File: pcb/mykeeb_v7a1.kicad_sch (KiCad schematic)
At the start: 71 parts, among them SW43 SW_Push, SW44 SW_SPDT, U1 74HC595, U2 xiao-ble

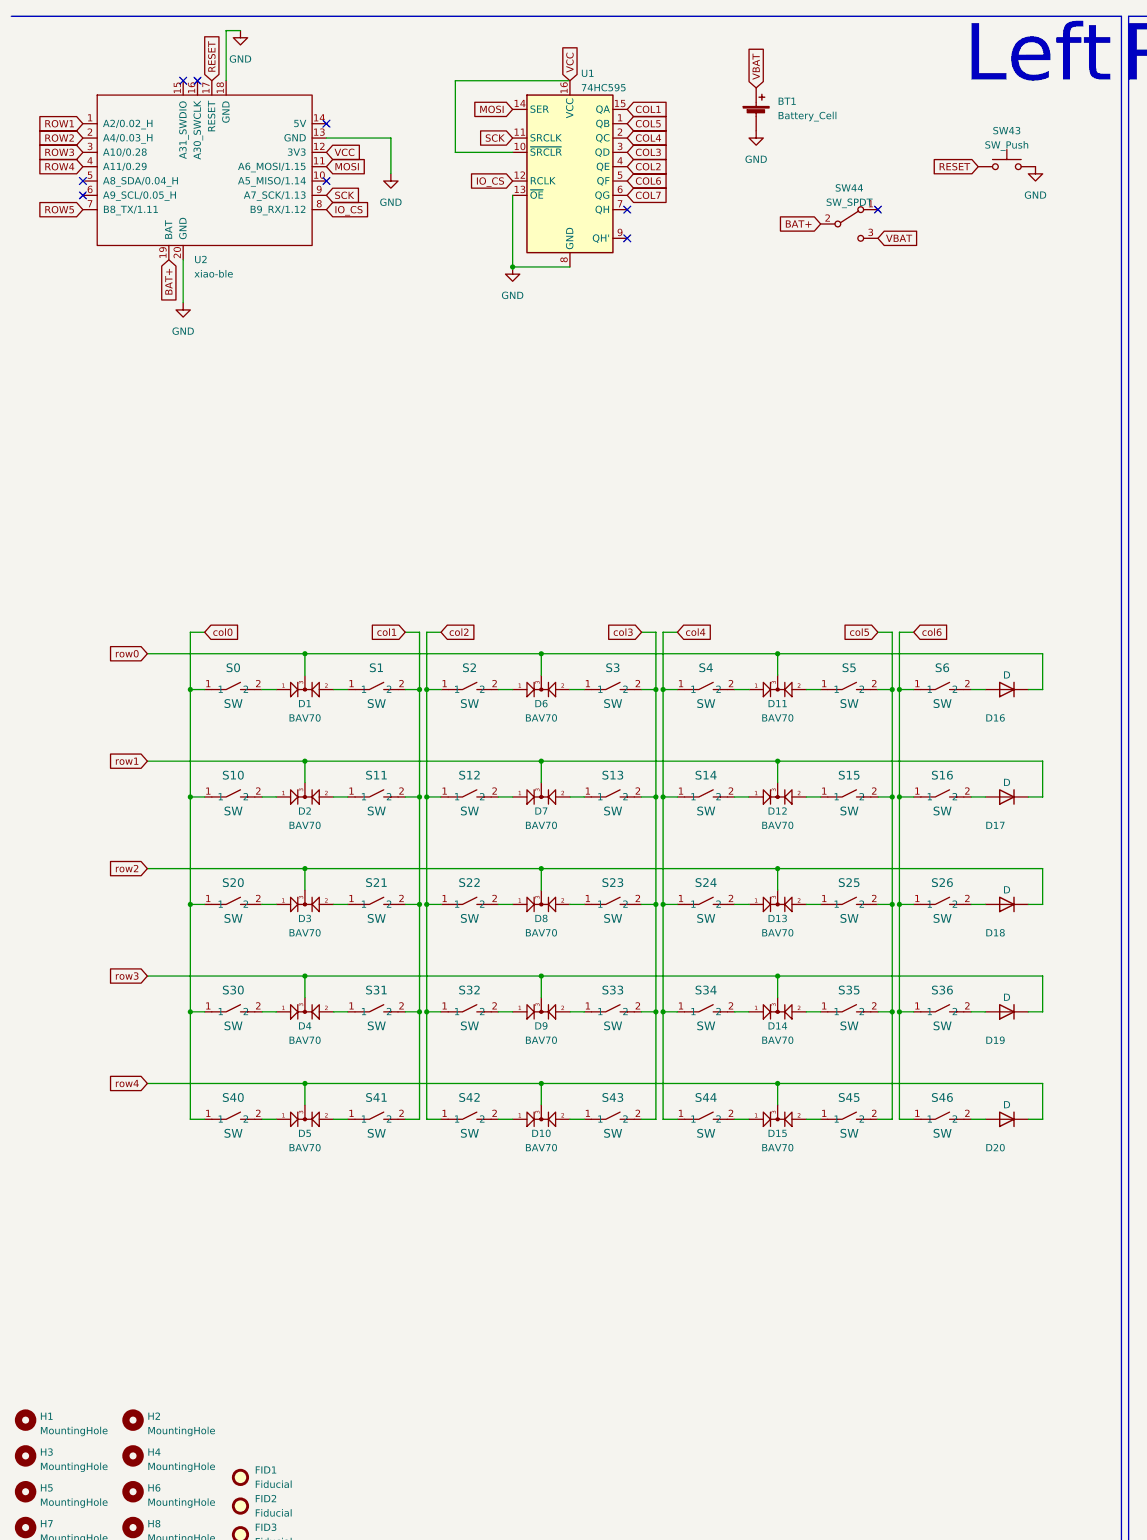
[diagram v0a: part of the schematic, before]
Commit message: wip
Signed-off-by: Maximilian Huber <gh@maxhbr.de>
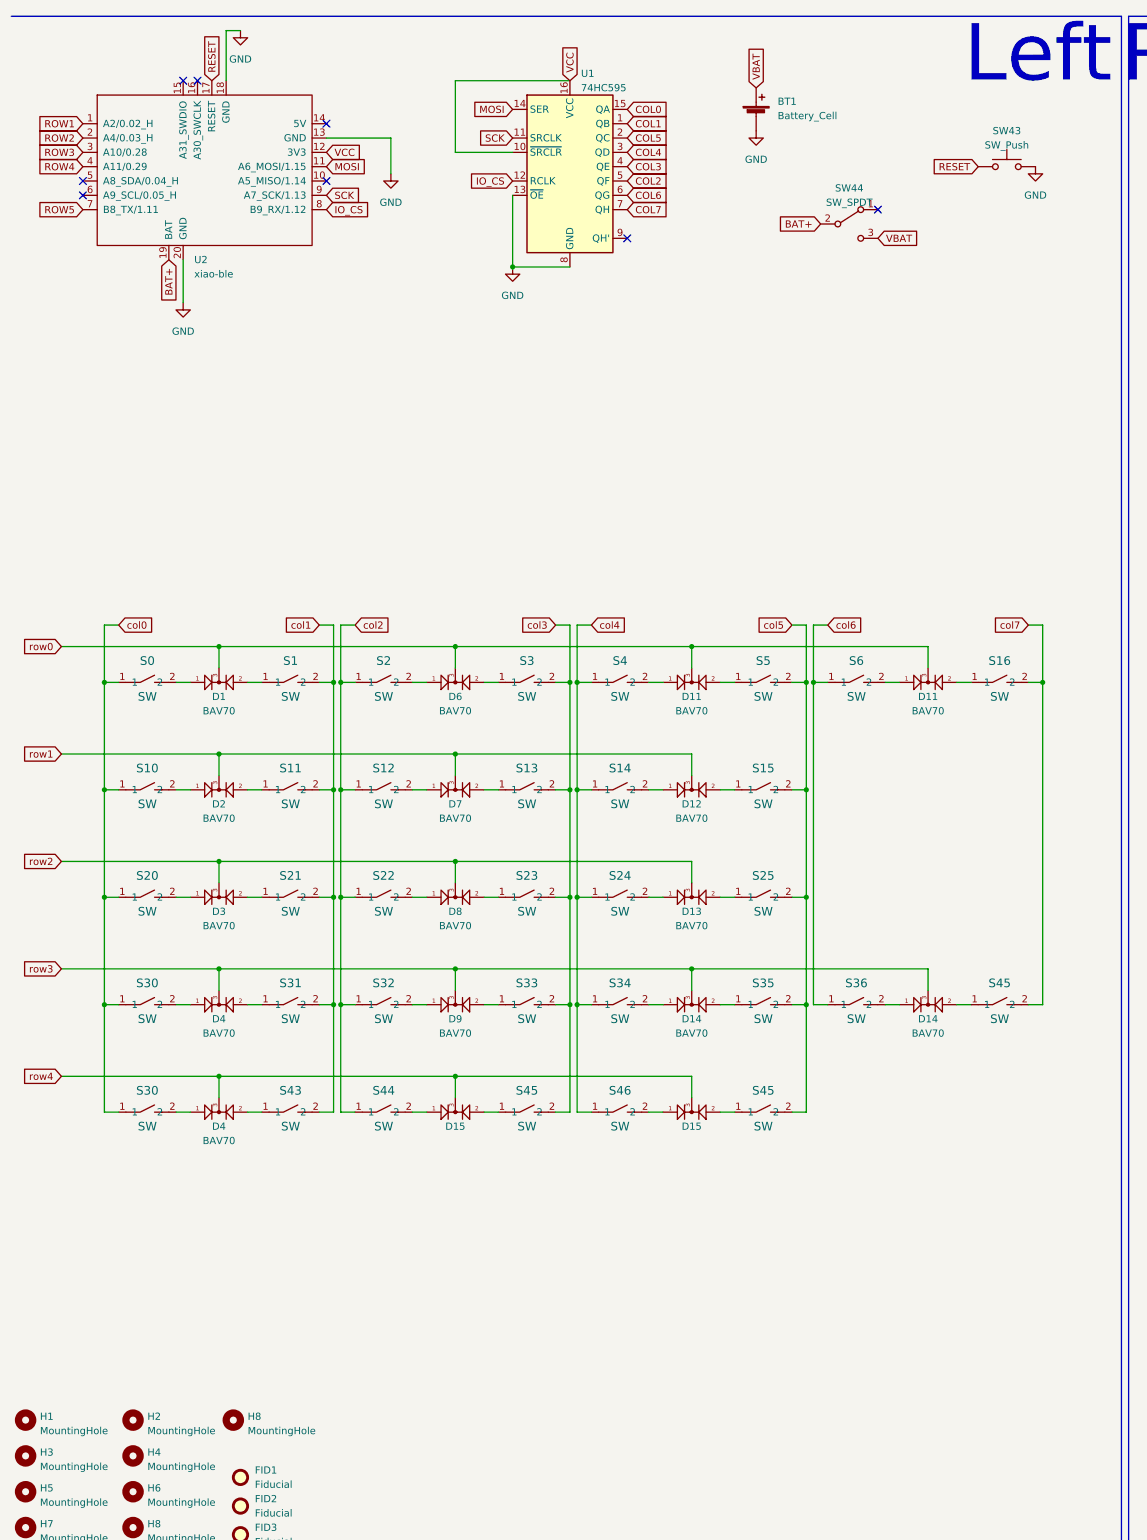
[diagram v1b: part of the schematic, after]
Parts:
- removed D10, D5: BAV70, mykeeb:SOT-23, symbol hillside_basic:BAV70_Small
- removed D16, D17, D18, D19, D20: D, mykeeb:D3_SMD, symbol Device:D
- removed S26, S40, S41, S42: SW, mykeeb:MX_KAILH_SOCKET_1U, symbol YAEMK:MX_1U
- added D11, D14, D15, D4: BAV70, Package_TO_SOT_SMD:SOT-23, symbol hillside_basic:BAV70_Small
- added H8: MountingHole, MountingHole:MountingHole_2.2mm_M2_DIN965, symbol Mechanical:MountingHole
- added S30, S45 (x2): SW, pretty:MX-1U-Hotswap, symbol YAEMK:MX_1U
- D1, D11, D12, D13, D14, D15, D2, D3, D4, D6, D7, D8, D9: footprint mykeeb:SOT-23 -> Package_TO_SOT_SMD:SOT-23
- S0, S1, S10, S11, S12, S13, S14, S15, S16, S2, S20, S21, S22, S23, S24, S25, S3, S30, S31, S32, S33, S34, S35, S36, S4, S43, S44, S45, S46, S5, S6: footprint mykeeb:MX_KAILH_SOCKET_1U -> pretty:MX-1U-Hotswap
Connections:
- net COL1: now also U1.1 (QB); no longer U1.15 (QA)
- net COL2: now also U1.5 (QF); no longer U1.4 (QE)
- net COL3: now also U1.4 (QE); no longer U1.3 (QD)
- net COL4: now also U1.3 (QD); no longer U1.2 (QC)
- net COL5: now also U1.2 (QC); no longer U1.1 (QB)
- net COL6: now also U1.6 (QG); no longer U1.5 (QF)
- net COL7: now also U1.7 (QH); no longer U1.6 (QG)
- net col0: now also S30.1
- net col1: now also S43.2
- net col2: now also S44.1
- net col3: now also S45.2; no longer S43.2
- net col4: now also S46.1; no longer S44.1
- net col5: now also S45.2; no longer S45.2
- net col6: no longer S16.1, S46.1
- net row0: now also D11.3 (K)
- net row3: now also D14.3 (K)
- net row4: now also D15.3 (K), D4.3 (K)
- net at S36.2: now also D14.1 (A1)
- net at S46.2: now also D15.1 (A1)
- net at S6.2: now also D11.1 (A1)
- net col7: now reaches S16.2
- net col7: now also S45.2
- net at S43.1: now also D4.2 (A2)
- new net: D4.1 (A1), S30.2
- new net: D11.2 (A2), S16.1
- new net: D14.2 (A2), S45.1
- new net: D15.2 (A2), S45.1
- new net COL0: U1.15 (QA)
- no-connect marks 9 -> 8
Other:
- moved on the sheet: D1, D11, D12, D13, D14, D15, D2, D3, D4, D6, D7, D8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
